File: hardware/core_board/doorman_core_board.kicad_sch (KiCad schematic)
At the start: 62 parts, among them J1 USB-C Connector, J10 VCC Test Pad, J2 Screw Terminals, J3 3V3 Test Pad, J4 Extension Board Connector, J5 Siedle BUS RX Test Pad, J6 BUS Test Pad, J7 BUS RX Test Pad, J8 TX Test Pad, J9 RX Test Pad, Q1 BC847BPN, Q2 BC817-40, Q3 BC817-40, Q4 BC817-40, Q6 BC847BPN, SW1 Button, SW2 Button, U2 AP63203WU, U3 GAQY252G3S, U4 ESP32-S3-MINI-1

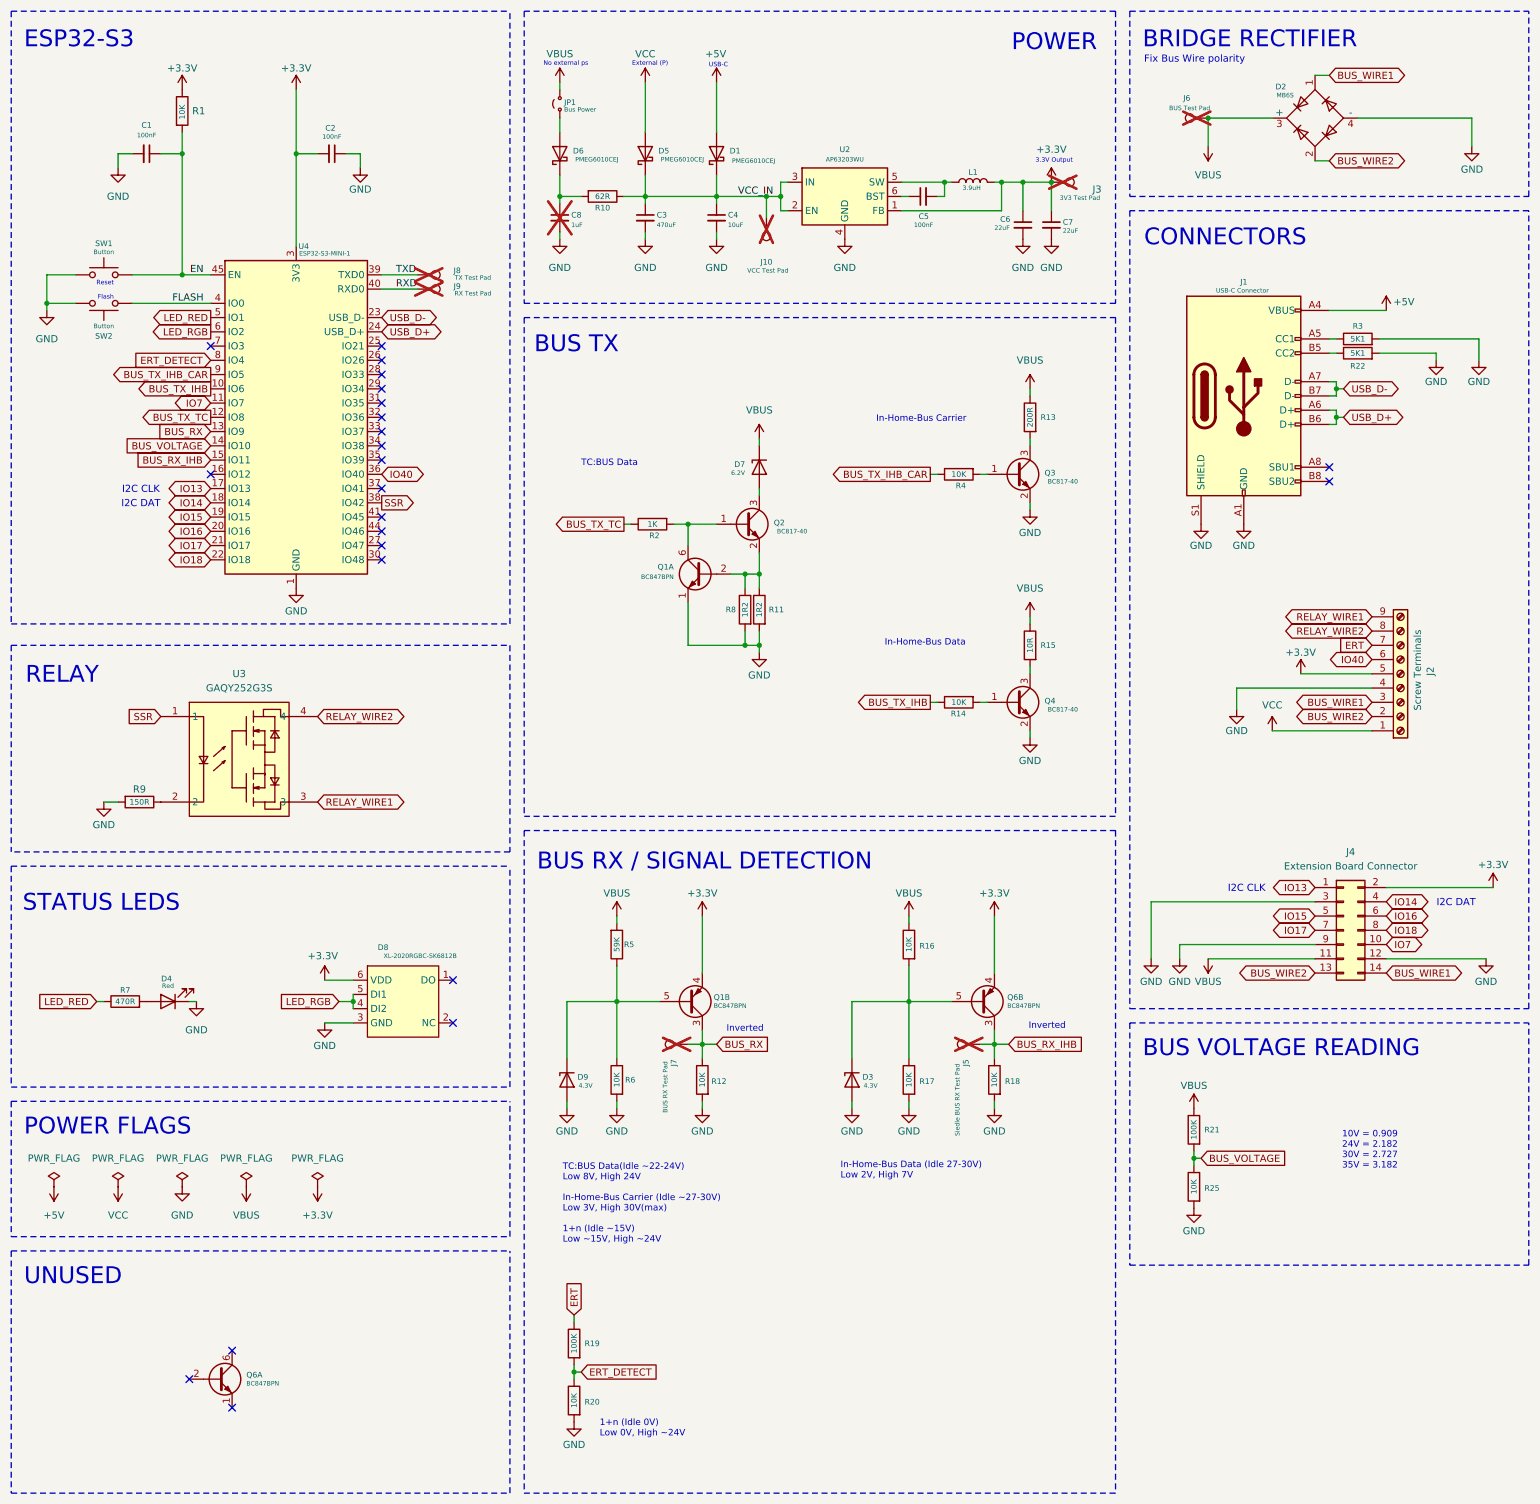
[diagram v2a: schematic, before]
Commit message: chore: Update pcb files core board 2.2.0
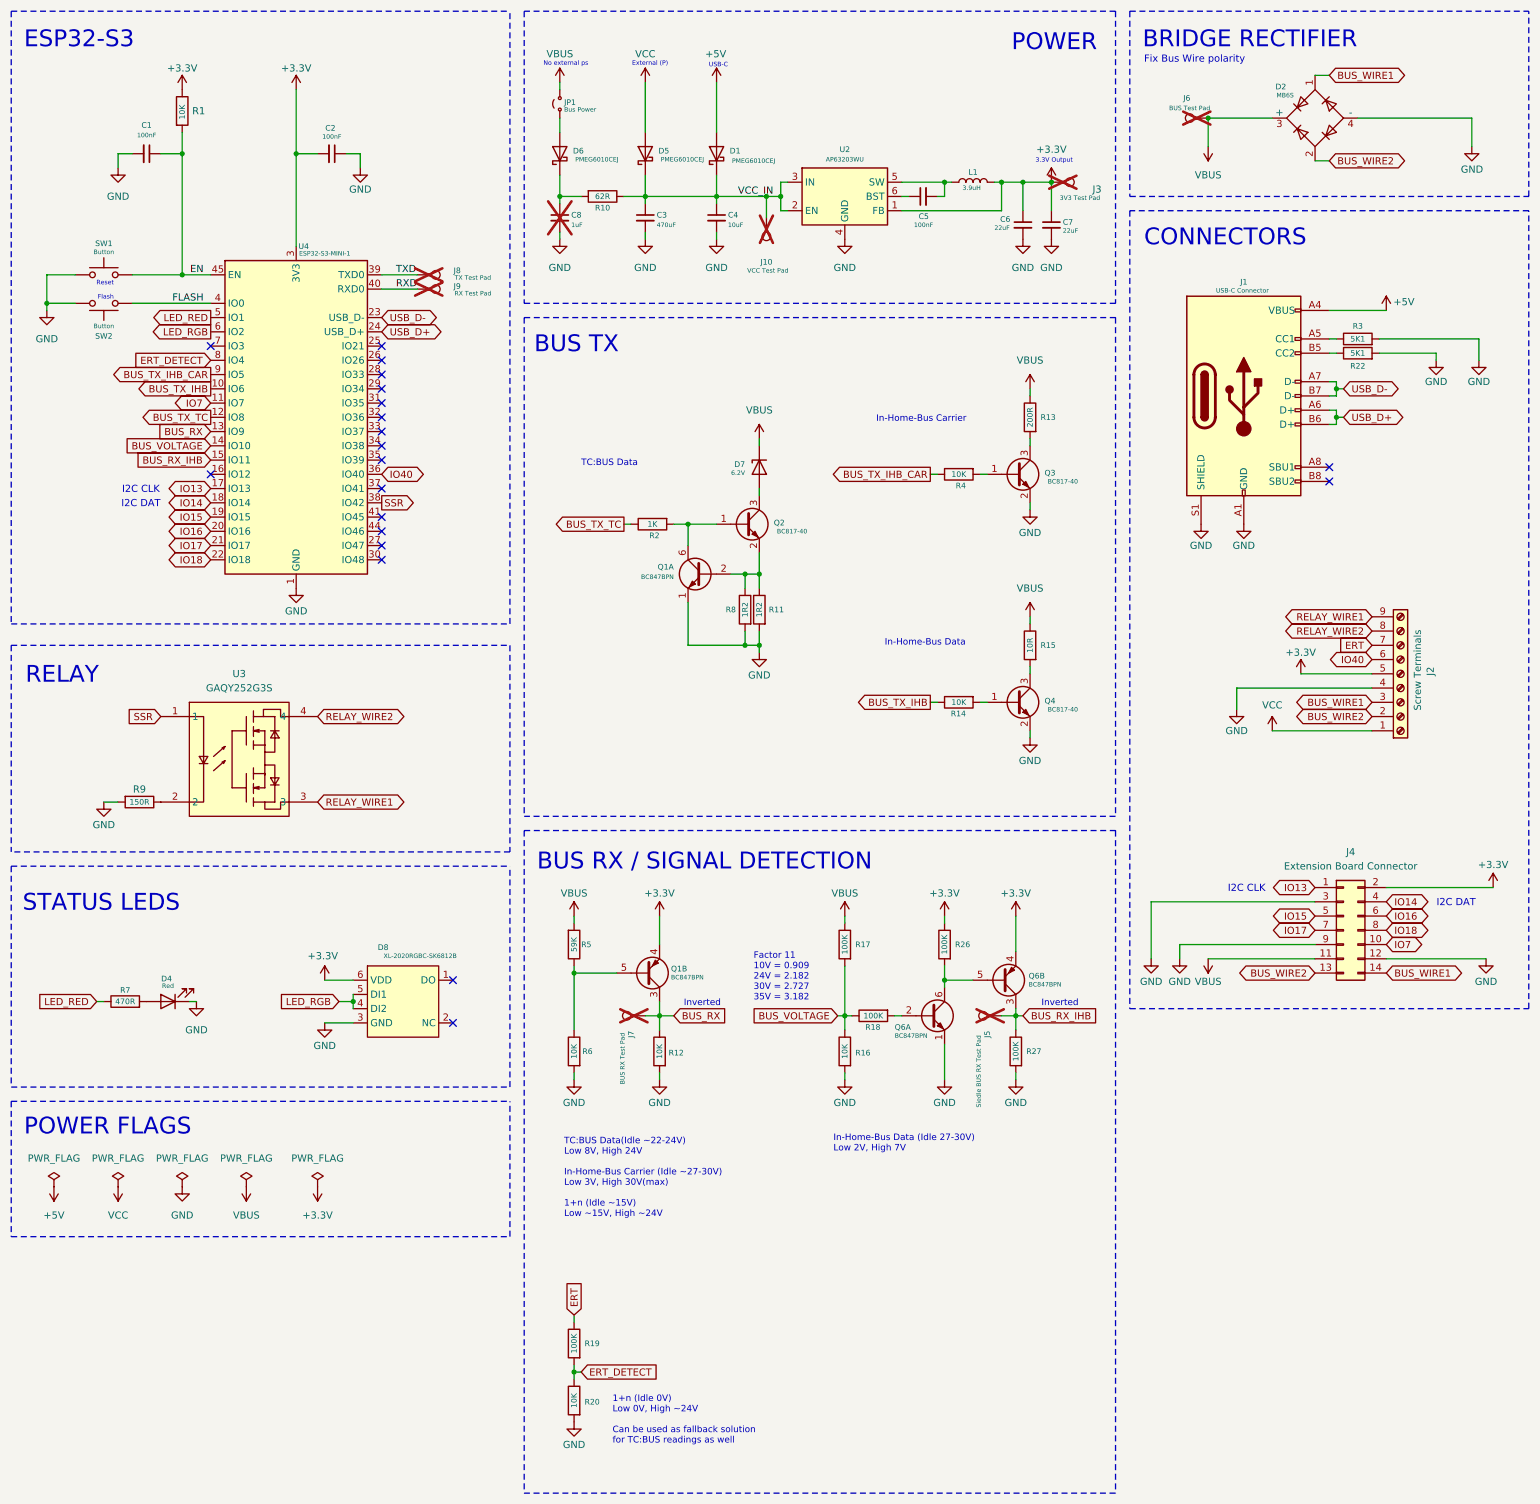
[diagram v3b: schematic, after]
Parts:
- removed D3, D9: 4.3V, Diode_SMD:D_SOD-123, symbol Diode:BZV55C6V2
- removed R21: 100K, Resistor_SMD:R_0603_1608Metric, symbol Device:R
- removed R25: 10K, Resistor_SMD:R_0603_1608Metric, symbol Device:R
- added R26, R27: 100K, Resistor_SMD:R_0603_1608Metric, symbol Device:R
- R10: LCSC C17971 -> C5576393; MPN 1206W4F620JT5E -> AC1206FR-7W62RL
- R15: LCSC C511457 -> C873921; MPN CRCW120610R0FKEAHP -> SR1206FR-7T10RL
- R17, R18: value 10K -> 100K; LCSC C25804 -> C25803; MPN 0603WAF1002T5E -> 0603WAF1003T5E
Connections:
- net +3.3V: now also R26.1
- net BUS_RX_IHB: now also R27.1; no longer R18.1
- net BUS_VOLTAGE: now also R16.1, R17.2, R18.1
- net GND: now also Q6.1 (E1), R16.2, R27.2; no longer R17.2, R18.2
- net VBUS: now also R17.1; no longer R16.1
- net at Q6.2 (B1): now also R18.2
- net at Q6.6 (C1): now also Q6.5 (B2), R26.2
- no-connect marks 23 -> 20
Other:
- note added: "1+n (Idle 0V) Low 0V, High ~24V Can be used as fallback solution for TC:BUS readings as well"
- note added: "Factor 11 10V = 0.909 24V = 2.182 30V = 2.727 35V = 3.182"
- note removed: "1+n (Idle 0V) Low 0V, High ~24V"
- note removed: "10V = 0.909 24V = 2.182 30V = 2.727 35V = 3.182"
- note removed: "BUS VOLTAGE READING"
- note removed: "UNUSED"
- moved on the sheet: J5, J7, Q1B, Q6A, Q6B, R12, R16, R5, R6

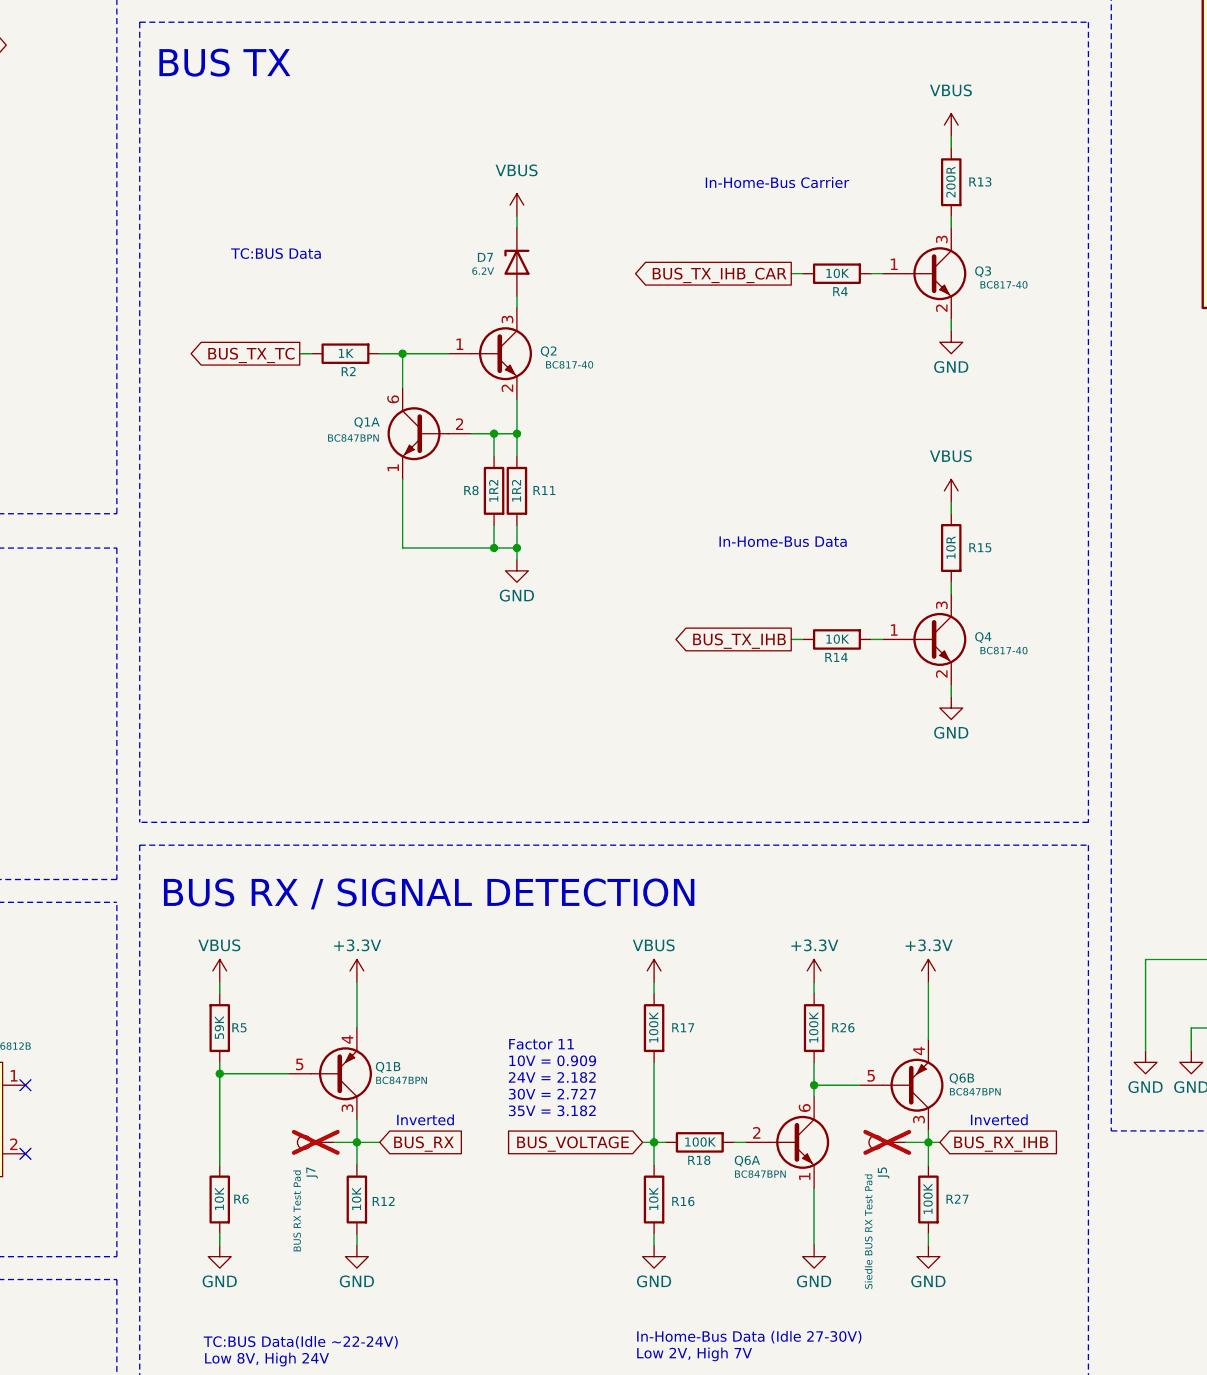
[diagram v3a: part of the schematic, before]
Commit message: chore: Update PCB files 2.2.0
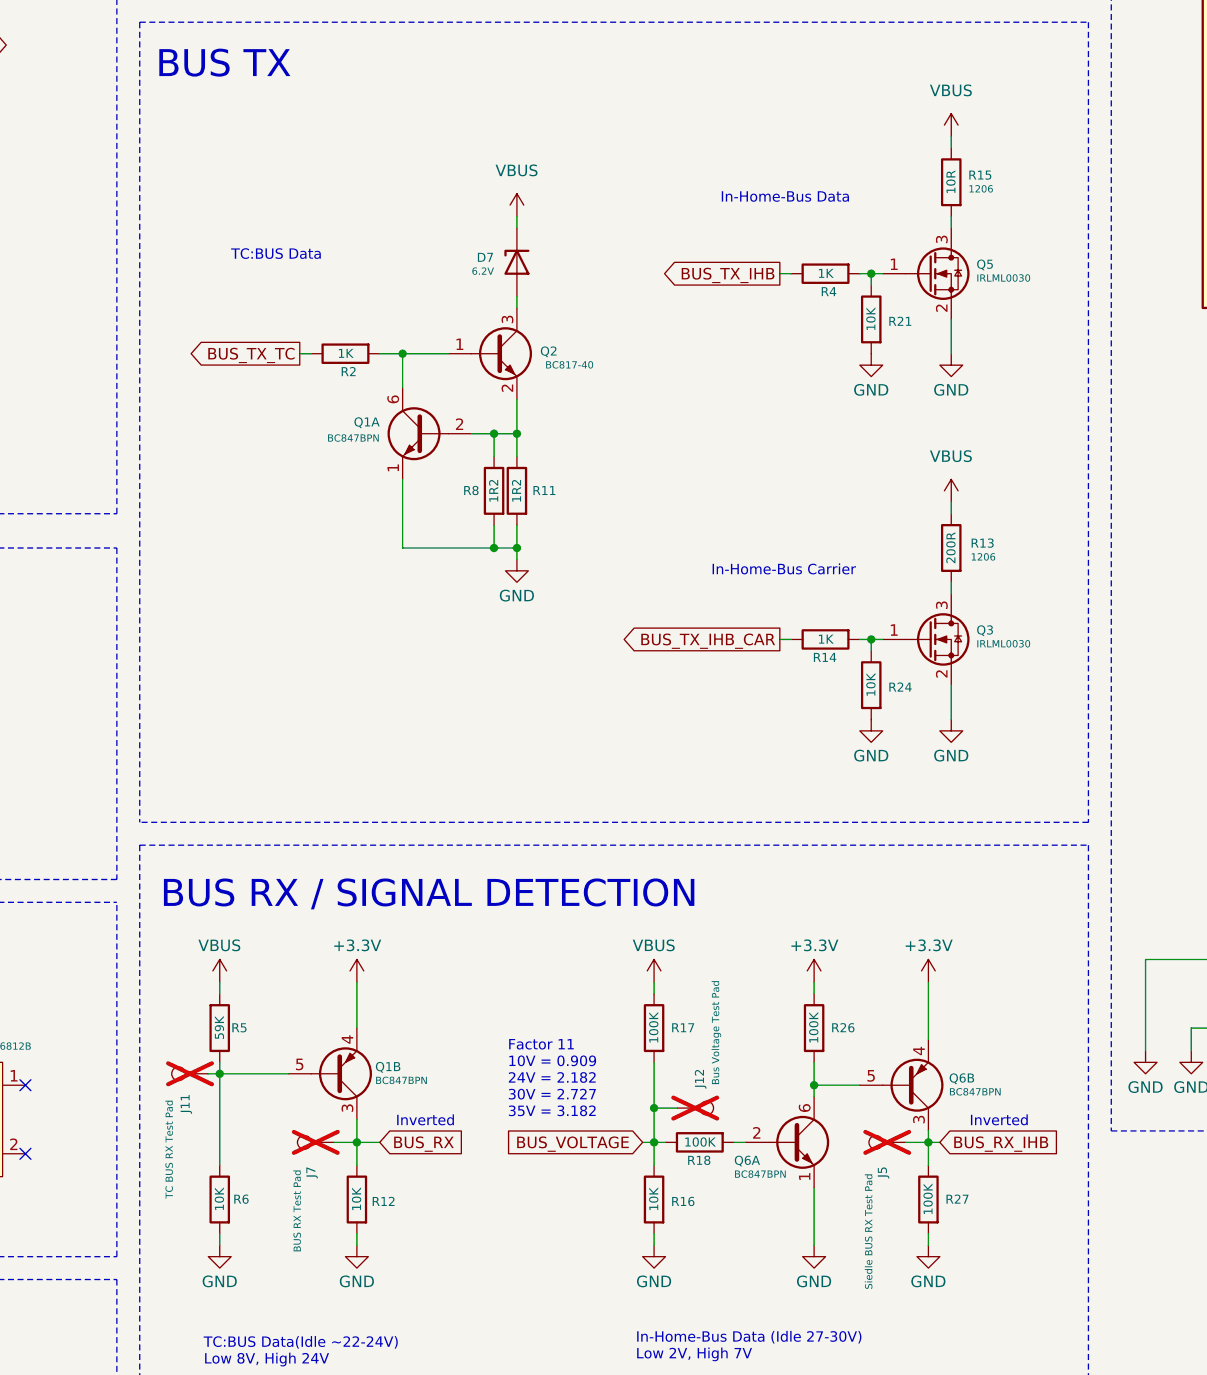
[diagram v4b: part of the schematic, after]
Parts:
- removed Q3, Q4: BC817-40, Package_TO_SOT_SMD:SOT-23, symbol Transistor_BJT:BC817
- added J11: TC BUS RX Test Pad, TestPoint:TestPoint_Pad_D1.0mm, symbol Connector:TestPoint
- added J12: Bus Voltage Test Pad, TestPoint:TestPoint_Pad_D1.0mm, symbol Connector:TestPoint
- added Q3, Q5: IRLML0030, Package_TO_SOT_SMD:SOT-23, symbol Transistor_FET:IRLML0030
- added R21, R24: 10K, Resistor_SMD:R_0603_1608Metric, symbol Device:R
- R14, R4: value 10K -> 1K; footprint Resistor_SMD:R_0603_1608Metric -> Resistor_SMD:R_0402_1005Metric; LCSC C25804 -> C11702; MPN 0603WAF1002T5E -> 0402WGF1001TCE; Package 0603 -> 0402
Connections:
- net BUS_TX_IHB: now also R4.1; no longer R14.1
- net BUS_TX_IHB_CAR: now also R14.1; no longer R4.1
- net BUS_VOLTAGE: now also J12.1
- net GND: now also Q3.2 (S), Q5.2 (S), R21.2, R24.2
- net at R4.2: now also Q5.1 (G), R21.1
- net at Q1.5 (B2), R5.1, R6.1: now also J11.1
- net at R13.2: now also Q3.3 (D)
- net at R15.2: now also Q5.3 (D)
- net at R14.2: now also Q3.1 (G), R24.1
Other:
- moved on the sheet: R13, R15
